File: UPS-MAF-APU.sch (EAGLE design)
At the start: 32 parts, among them J1 CONNECTOR_PI_40_PIN, J2 Barrel DC In, J3 OLED, J4 OSTOQ045451, J5 External DS18B20 Temp, J6 FTDI Serial Console, J7 MagJack, U1 OLED_I2C, U2 SI7006-A20-IM, U4 INA260AIPW, U6 ENC28J60_SS, U7 5V SMPS, Y1 ECS-250-20-3X-EN-TR

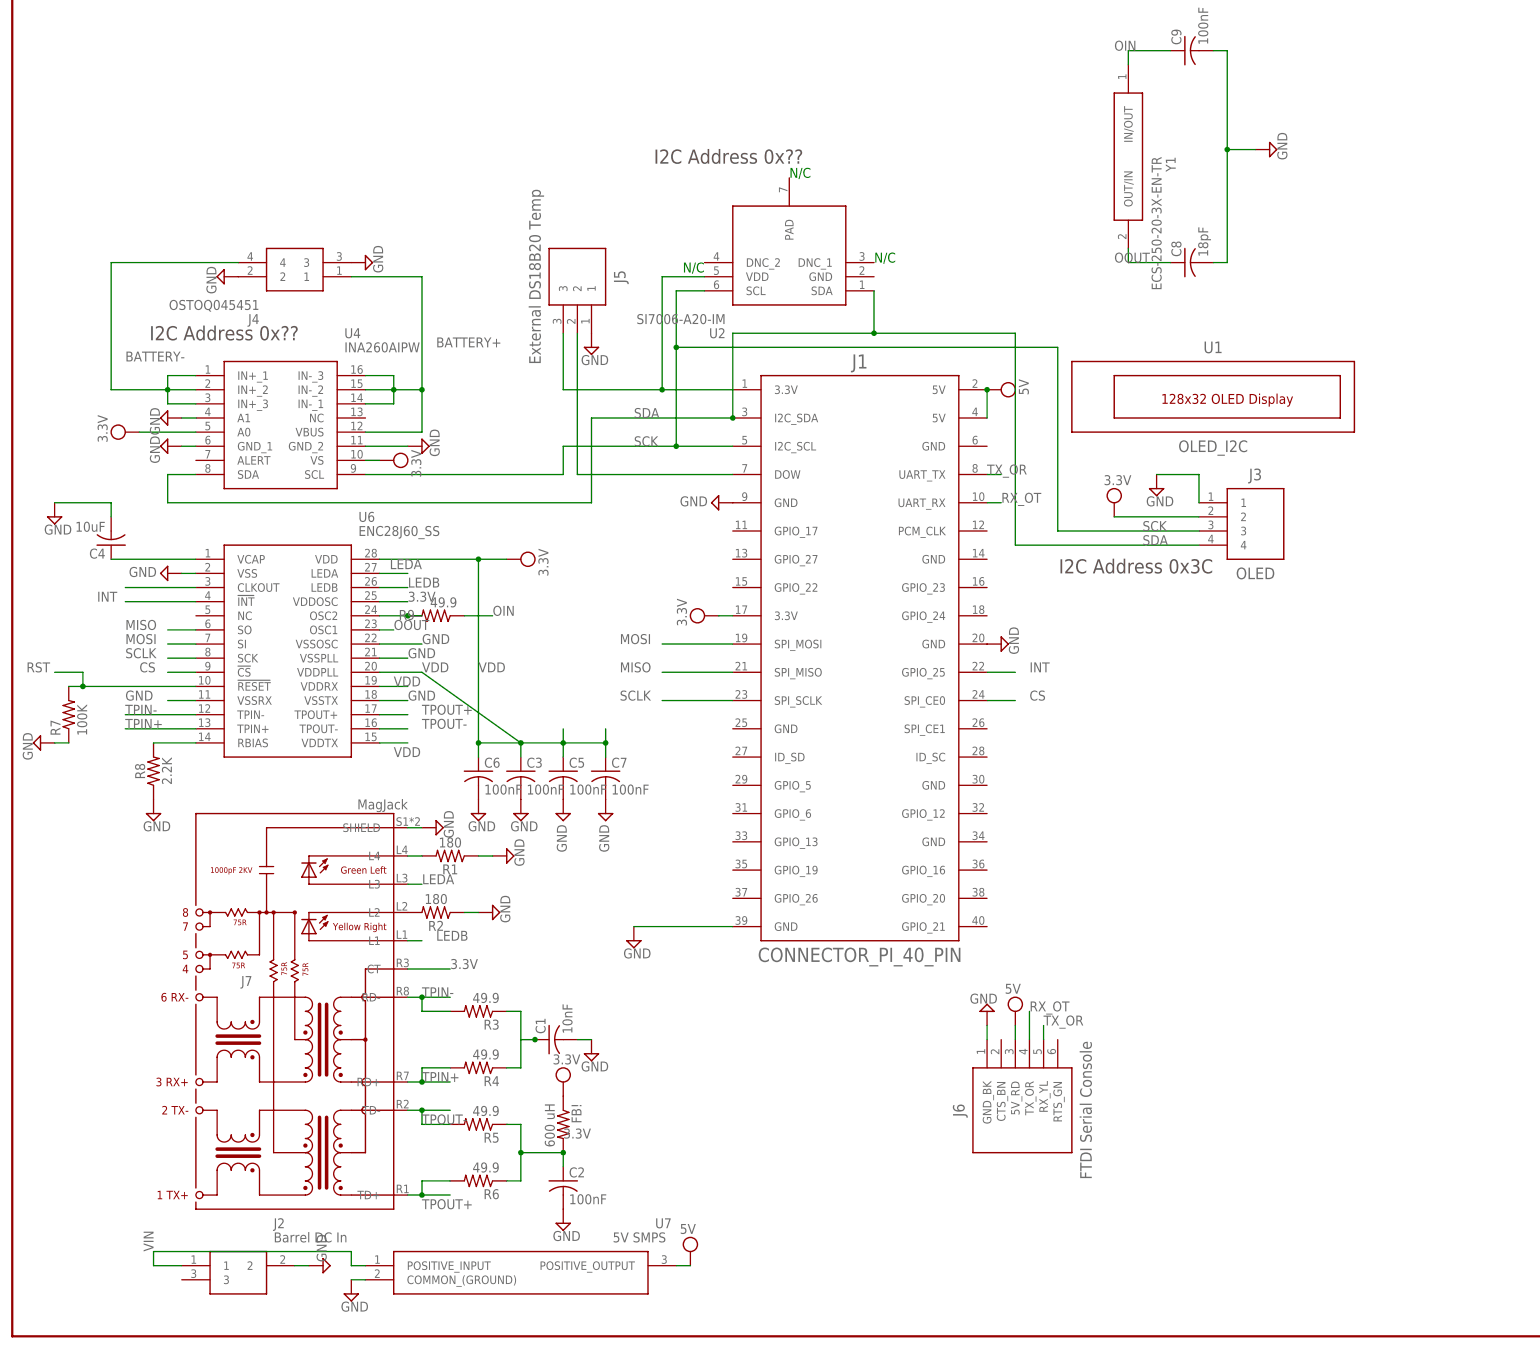
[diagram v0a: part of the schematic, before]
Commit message: README
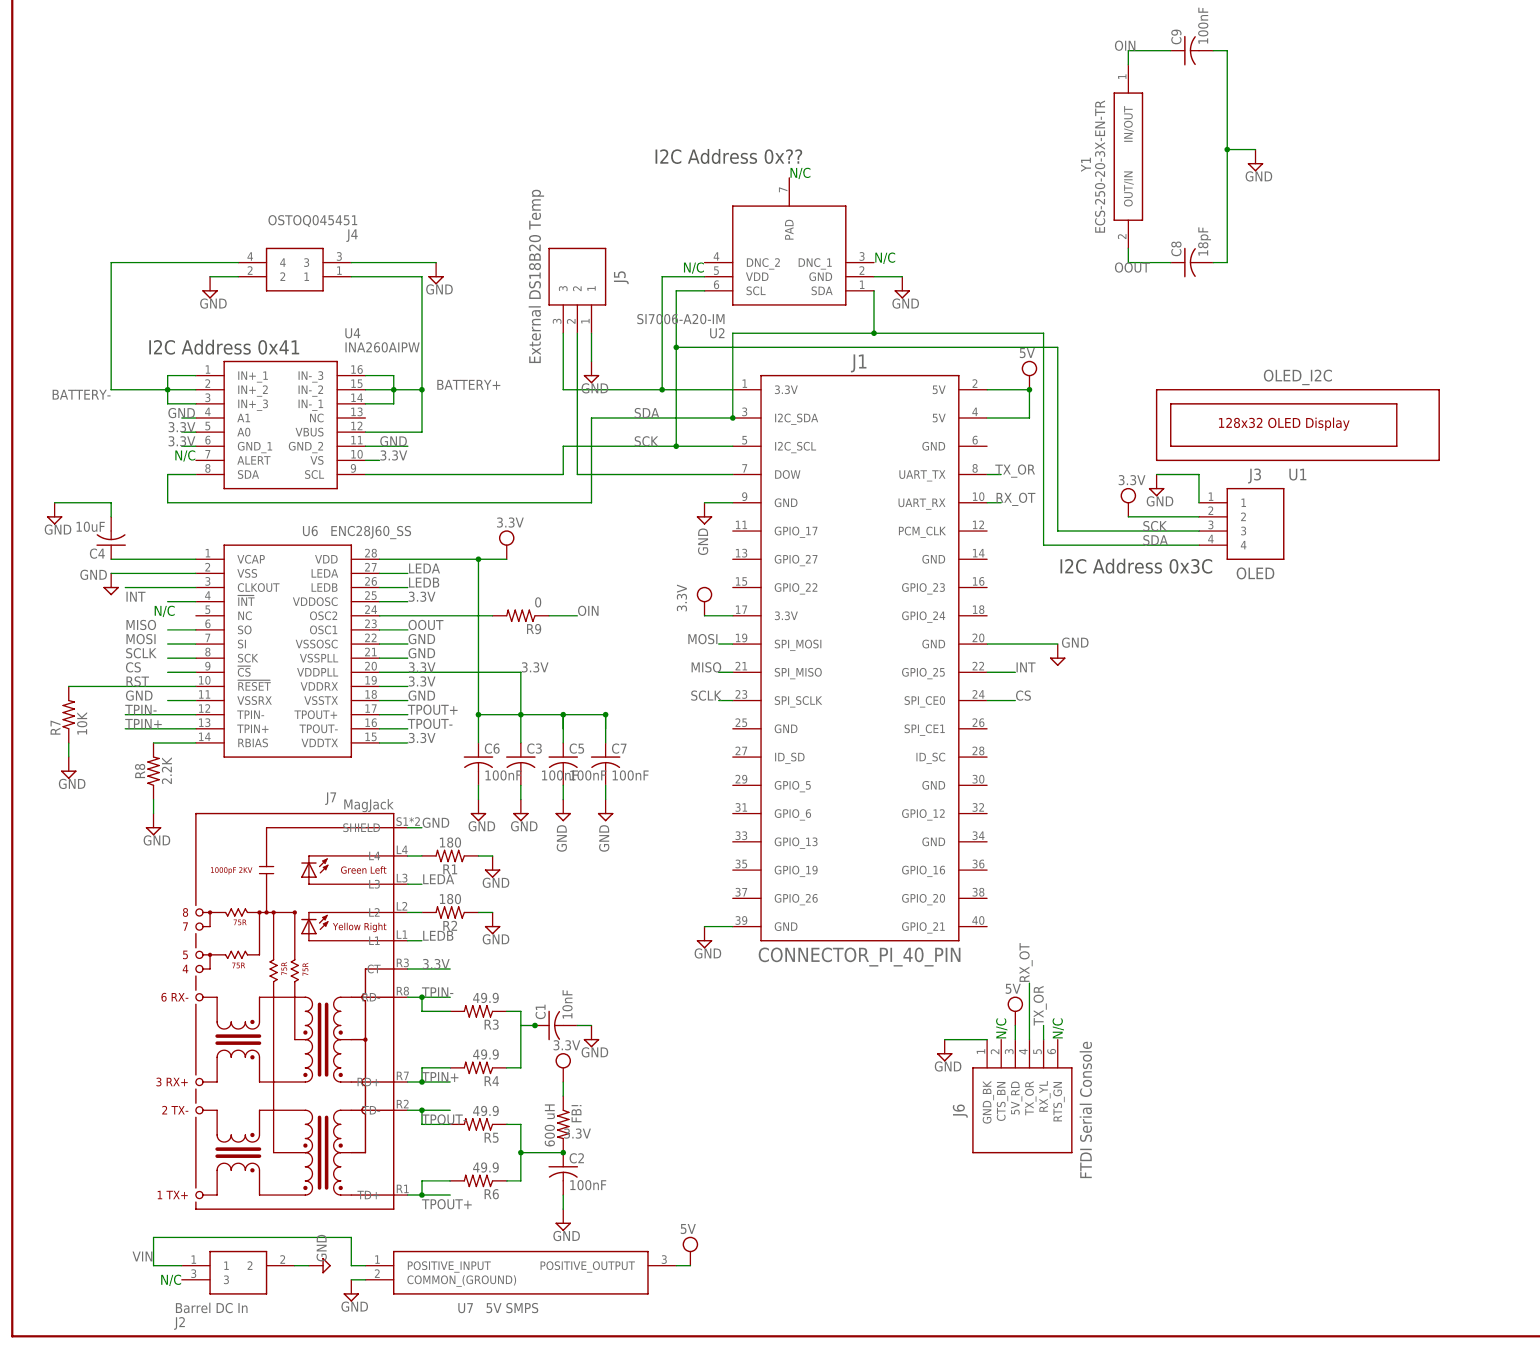
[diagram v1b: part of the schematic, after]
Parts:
- R7: value 100K -> 10K
- R9: value 49.9 -> 0
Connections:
- removed net VDD: C3.1, C5.1, C6.1, C7.1, U6.VDD, U6.VDDPLL, U6.VDDRX, U6.VDDTX
- net 3.3V: now also C3.1, C5.1, C6.1, C7.1, U4.GND_1, U6.VDD, U6.VDDPLL, U6.VDDRX, U6.VDDTX
- net GND: now also U2.GND; no longer U4.GND_1
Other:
- note added: "I2C Address 0x41"
- note removed: "add battery/charger connector add power, status lights"
- moved on the sheet: C1, C2, C3, C5, C6, C7, R2, R9, U1
